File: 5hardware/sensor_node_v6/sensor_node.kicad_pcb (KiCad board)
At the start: 2 copper layers, 48 x 47 mm, 71 parts, among them J1 USB_C_Receptacle_USB2.0, J2 PJ-320D-A, J3 Conn_01x18_Socket, J4 Conn_01x18_Socket, J5 Conn_01x04_Pin, P1 S3B-PH-SM4-TB, Q1 BC818, Q2 Si2371EDS, Q3 AO3400A, Q4 Si2371EDS, Q5 Si2371EDS, SW1 SW_Push, SW2 RotaryEncoder, SW3 SW_Push, SW4 SW_Push, SW5 SW_Push, SW7 SW_Push, U1 INA219AxD, U12 APDS-9960, U13 SHT31-DIS, U15 DS1307Z+, U16 DS3231M, U17 BH1750FVI-TR, U2 ESP-12F, U4 CH32V003F4P6, U7 XC6206PxxxMR, U8 TPL5110, Y1 Crystal, Y2 Crystal

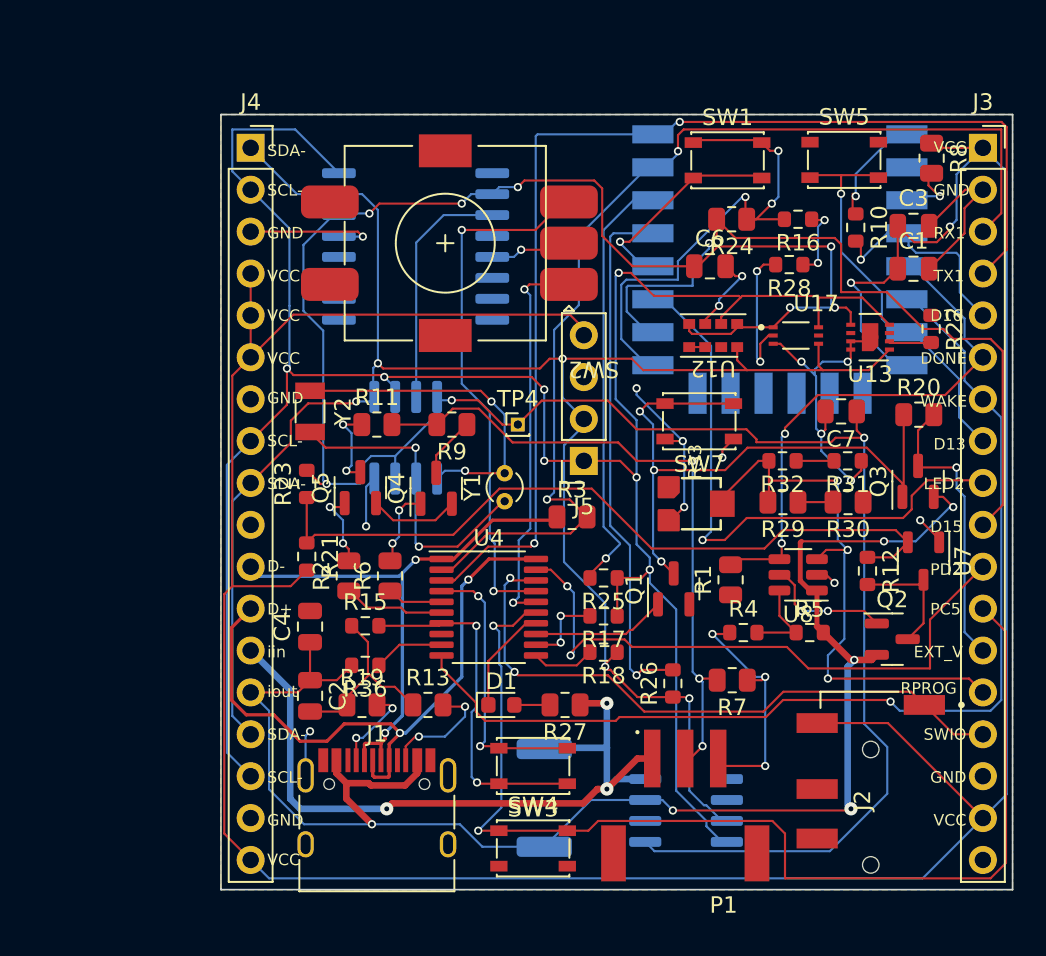
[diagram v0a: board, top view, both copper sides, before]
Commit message: update PCB v8.0
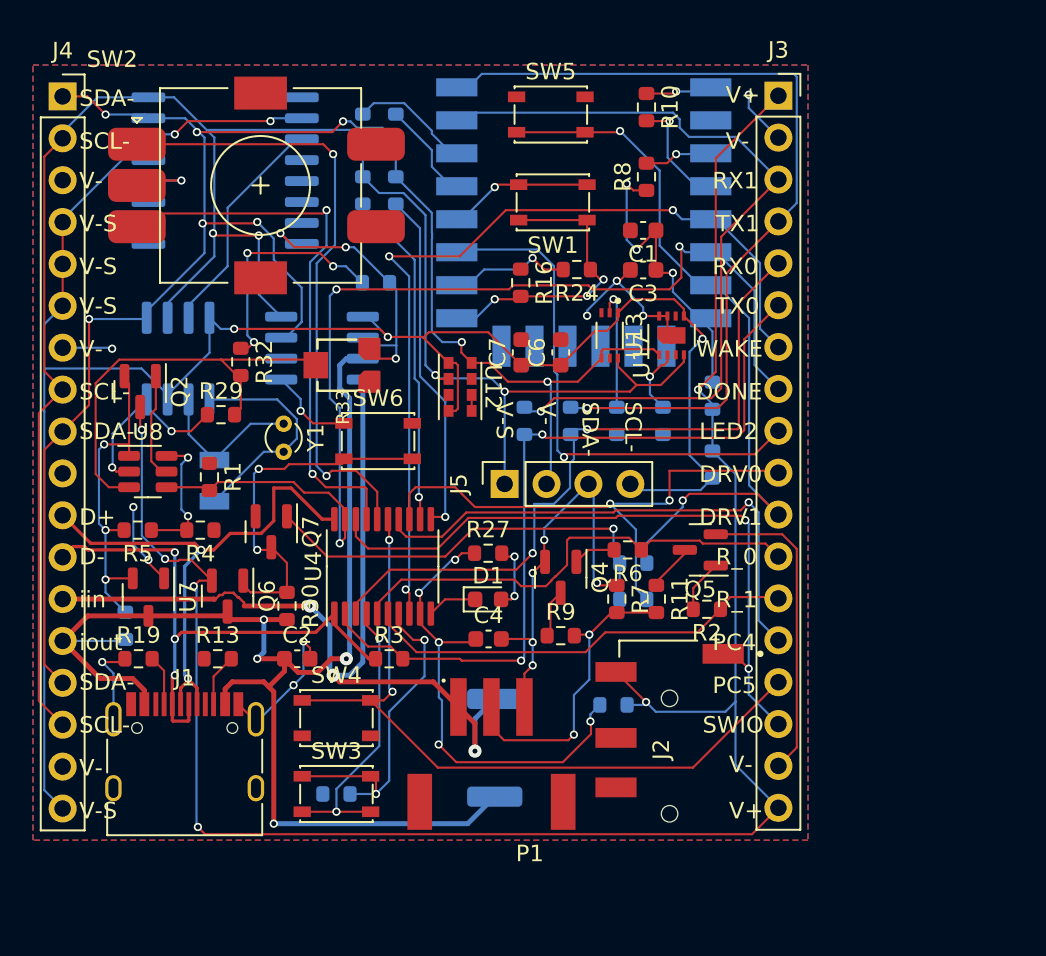
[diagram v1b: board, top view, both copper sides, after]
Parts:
- removed Q1: BC818, Package_TO_SOT_SMD:SOT-23
- removed Q3: AO3400A, Package_TO_SOT_SMD:SOT-23
- removed SW7: SW_Push, Button_Switch_SMD:SW_SPST_PTS810
- removed TP4: TestPoint, Connector_PinHeader_1.00mm:PinHeader_1x01_P1.00mm_Vertical
- added Q6: AO3400A, Package_TO_SOT_SMD:SOT-23, F.Cu at (151.6, 72.2)
- added Q7: BC818, Package_TO_SOT_SMD:SOT-23, F.Cu at (154.2, 68.3)
- added R34: R, Resistor_SMD:R_0603_1608Metric, B.Cu at (176.2, 70.2)
- added R35: R, Resistor_SMD:R_0603_1608Metric, B.Cu at (169.6, 61.6)
- added R37: R, Resistor_SMD:R_0603_1608Metric, B.Cu at (172.4, 61.6)
- added SW6: SW_Push, Button_Switch_SMD:SW_SPST_PTS810, F.Cu at (160.7, 62.8)
- C1, C2, C3, C4, C6, C7: footprint Capacitor_SMD:C_0805_2012Metric -> Capacitor_SMD:C_0603_1608Metric
- R1, R11, R13, R19, R2, R24, R27, R29, R3, R30, R6, R7, R8, R9: footprint Resistor_SMD:R_0805_2012Metric -> Resistor_SMD:R_0603_1608Metric
- R12, R15, R17, R18, R21, R22, R23, R25, R26, R28, R31, R36, Y2: moved to B.Cu
- R20: footprint Resistor_SMD:R_0805_2012Metric -> Resistor_SMD:R_0603_1608Metric; moved to B.Cu
- moved Q2 48.0 mm to (146.3, 59.8), turned to -90 degrees
- moved U7 47.1 mm to (146.8, 72.3)
- moved R12 45.1 mm to (145.4, 74.0)
- moved R5 41.2 mm to (146.2, 68.2), turned to 180 degrees
- moved U8 39.9 mm to (146.8, 64.7), turned to 0 degrees
- moved R26 37.7 mm to (161.8, 43.8)
- moved U1 35.7 mm to (157.3, 57.2), turned to 0 degrees
- moved R30 34.6 mm to (155.2, 72.8), turned to -90 degrees
- moved R29 34.5 mm to (151.2, 61.2), turned to 0 degrees
- moved SW2 34.2 mm to (144.6, 40.1), turned to 0 degrees
- moved R4 33.5 mm to (149.9, 68.2), turned to 180 degrees
- moved R32 33.4 mm to (152.4, 58.0), turned to -90 degrees
- moved R1 32.2 mm to (150.5, 65.0), turned to -90 degrees
- moved R25 31.0 mm to (159.8, 43.8), turned to 90 degrees
- moved R18 30.7 mm to (161.8, 47.6), turned to -90 degrees
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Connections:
- net LED02 renamed LED2
- C1 pad 1: VCC -> Net-(U2-VCC)
- C3 pad 1: VCC -> Net-(U2-VCC)
- C4 pad 1: iout -> Net-(U4-VDD)
- J2 pad 2: VCC -> +3.3V
- J3 pad 1: VCC -> +3.3V
- J3 pad 10: D15 -> DRIVE0
- J3 pad 11: PD2 -> DRIVE1
- J3 pad 12: PC5 -> R_0
- J3 pad 13: EXT_VCC -> R_1
- J3 pad 14: RPROG -> PC4
- J3 pad 15: SWIO -> PC5
- J3 pad 16: GND -> SWIO
- J3 pad 17: VCC -> GND
- J3 pad 18: unconnected-(J3-Pin_18-Pad18) -> +3.3V
- J3 pad 5: D16 -> RX0
- J3 pad 6: DONE -> TX0
- J3 pad 7: WAKE0 -> WAKE
- J3 pad 8: D13 -> DONE
- J4 pad 11: D- -> D+
- J4 pad 12: D+ -> D-
- J4 pad 18: VCC -> V-S
- J4 pad 4: VCC -> V-S
- J4 pad 5: VCC -> V-S
- J4 pad 6: VCC -> V-S
- J5 pad 4: VCC -> V-S
- Q2 pad 2: iout -> Net-(Q2-S)
- Q2 pad 3: Net-(Q2-D) -> +3.3V
- R12 pad 1: +3.3V -> Net-(Q2-S)
- R12 pad 2: Net-(Q2-D) -> iout
- R2 pad 1: Net-(U4-PA2) -> R_1
- R20 pad 1: Net-(Q1-C) -> DRIVE0
- R20 pad 2: EXT_VCC -> DRIVE-
- R21 pad 1: +3.3V -> Net-(U2-VCC)
- R21 pad 2: VCC -> +3.3V
- R23 pad 1: +3.3V -> V-S
- R23 pad 2: V-S -> +3.3V
- R27 pad 1: iin -> Net-(U4-VDD)
- R29 pad 1: Net-(R29-Pad1) -> GND
- R29 pad 2: RPROG -> Net-(U8-DELAY/M_DRV)
- R3 pad 2: RX1 -> TX0
- R30 pad 1: GND -> Net-(Q6-G)
- R30 pad 2: Net-(R29-Pad1) -> iout
- R32 pad 2: RPROG -> Net-(U8-DELAY/M_DRV)
- R33 pad 2: RPROG -> Net-(U8-DELAY/M_DRV)
- R36 pad 2: iout -> +3.3V
- R5 pad 2: iout -> Net-(Q2-S)
- R6 pad 1: Net-(U4-PA1) -> R_0
- R8 pad 1: VCC -> Net-(U2-VCC)
- SW5 pad 2: D13 -> DRIVE1
- U2 pad 5: DONE -> WAKE
- U2 pad 6: WAKE0 -> DONE
- U2 pad 7: D13 -> DRIVE1
- U2 pad 8: VCC -> Net-(U2-VCC)
- U4 pad 10: WAKE0 -> Net-(D1-K)
- U4 pad 13: Net-(Q1-B) -> DRIVE0
- U4 pad 14: Net-(D1-K) -> PC4
- U4 pad 19: PD2 -> DONE
- U4 pad 2: RX1 -> TX0
- U4 pad 3: TX1 -> RX0
- U4 pad 5: Net-(U4-PA1) -> R_0
- U4 pad 6: Net-(U4-PA2) -> R_1
- U4 pad 8: unconnected-(U4-PD0-Pad8) -> WAKE
- U7 pad 2: +3.3V -> Net-(Q2-S)
- U7 pad 3: Net-(Q2-D) -> iout
- U8 pad 1: iout -> Net-(Q2-S)
- U8 pad 3: RPROG -> Net-(U8-DELAY/M_DRV)
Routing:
- net VCC: track 189.3 -> 0.00 mm, vias 2 -> 0
- net +3.3V: track 45.3 -> 121.9 mm, vias 0 -> 6
- net WAKE0: track 65.1 -> 0.00 mm, vias 1 -> 0
- net WAKE: track 0.00 -> 52.9 mm, vias 0 -> 3
- net TX0: track 0.00 -> 48.0 mm, vias 0 -> 2
- net DRIVE1: track 0.00 -> 45.3 mm, vias 0 -> 2
- net RX0: track 0.00 -> 43.0 mm, vias 0 -> 2
- net Net-(Q1-C): track 39.2 -> 0.00 mm, vias 3 -> 0
- net D15: track 45.3 -> 6.72 mm
- net PD2: track 37.3 -> 0.00 mm, vias 2 -> 0
- net RPROG: track 35.6 -> 0.00 mm, vias 3 -> 0
- net DRIVE0: track 0.00 -> 33.3 mm, vias 0 -> 2
- net DONE: track 33.3 -> 65.4 mm, vias 2 -> 3
- net PC4: track 0.00 -> 32.0 mm, vias 0 -> 1
- net R_0: track 0.00 -> 28.7 mm
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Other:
- board outline removed
- board text added: "DRV0"
- board text added: "DRV1"
- board text added: "PC4"
- board text added: "RX0"
- board text added: "R_0"
- board text added: "R_1"
- board text added: "TX0"
- board text added: "V+"
- board text added: "V-"
- board text added: "V-S"
- board text removed: "D13"
- board text removed: "D15"
- board text removed: "D16"
- board text removed: "ESP-MESS BaseB V7.0 The Future is Now 01/31/24"
- board text removed: "EXT_V"
- board text removed: "GND"
- board text removed: "PD2"
- board text removed: "RPROG"
- board text removed: "VCC"
